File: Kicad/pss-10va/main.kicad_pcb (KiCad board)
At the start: 2 copper layers, 150 x 60 mm, 103 parts, among them K1 MAIN AC, K2 VCC, P1 2k, P2 2k, U1 LM317, U2 LM337, X101 LOGO

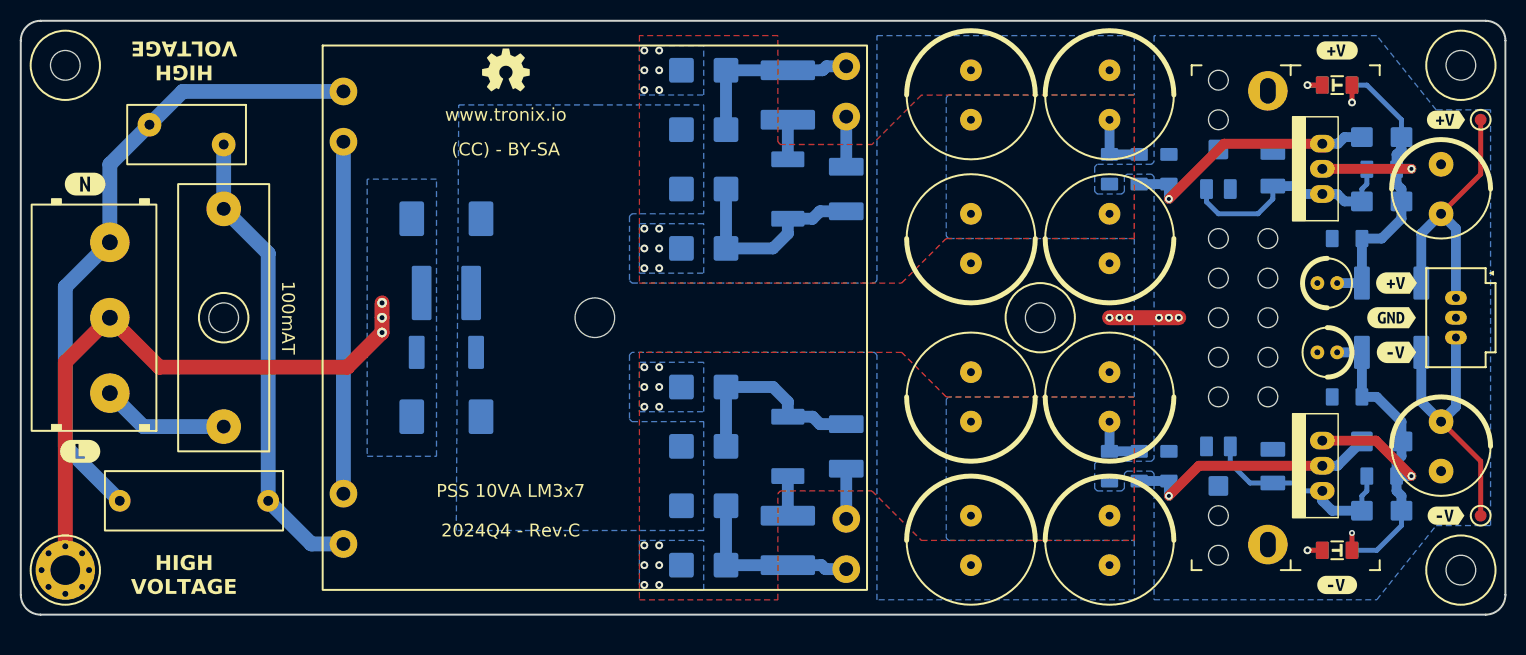
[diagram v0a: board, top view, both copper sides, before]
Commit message: Up
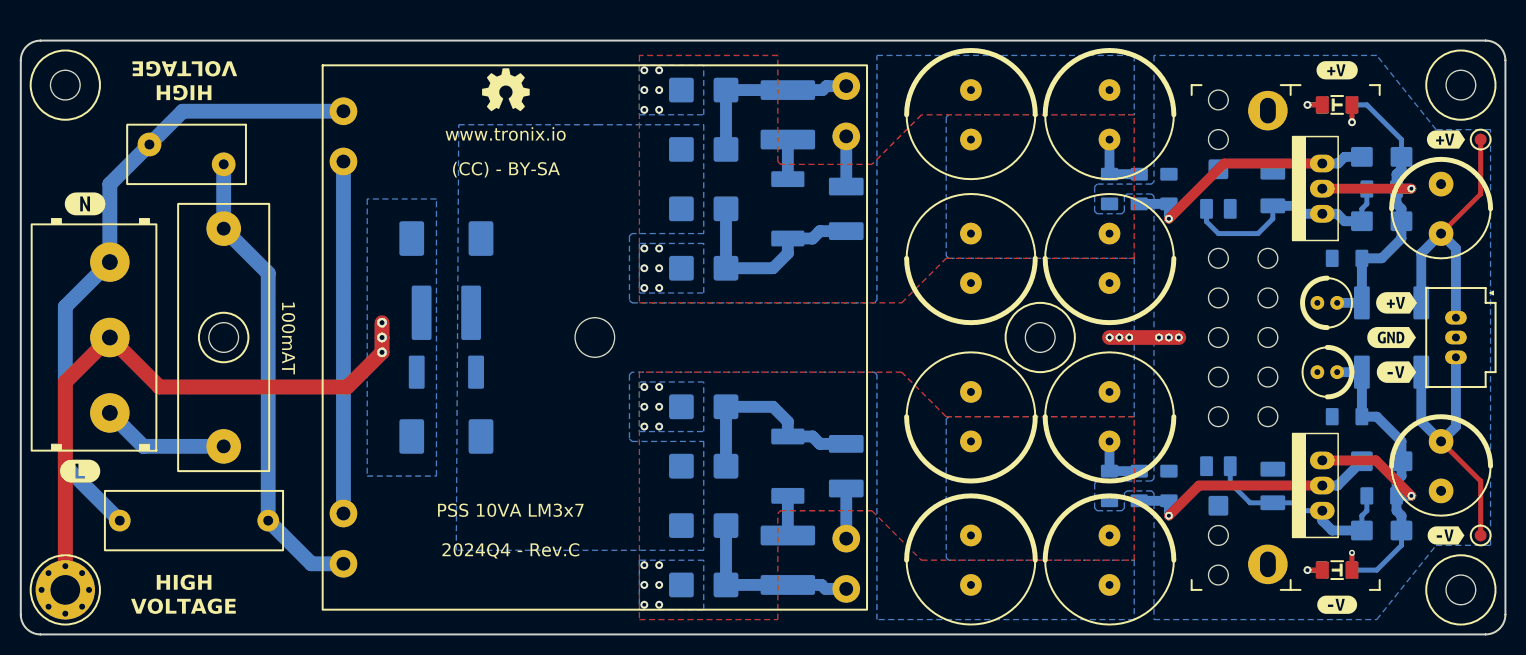
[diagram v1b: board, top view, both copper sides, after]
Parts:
- moved C1 2.00 mm to (92.5, 108.5)
- moved C10 2.00 mm to (185.0, 98.0)
- moved C11 2.00 mm to (185.0, 82.0)
- moved C12 2.00 mm to (185.0, 112.5)
- moved C13 2.00 mm to (185.0, 75.0)
- moved C14 2.00 mm to (185.0, 105.0)
- moved C15 2.00 mm to (191.0, 75.0)
- moved C16 2.00 mm to (191.0, 105.0)
- moved C17 2.00 mm to (201.5, 75.0)
- moved C18 2.00 mm to (201.5, 105.0)
- moved C19 2.00 mm to (209.0, 82.0)
- moved C2 2.00 mm to (118.0, 87.5)
- moved C20 2.00 mm to (209.0, 98.0)
- moved C21 2.00 mm to (207.0, 86.5)
- moved C22 2.00 mm to (207.0, 93.5)
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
